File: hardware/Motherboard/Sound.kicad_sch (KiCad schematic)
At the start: 2 parts, among them U29 74LS02, U65 AY-3-8910A

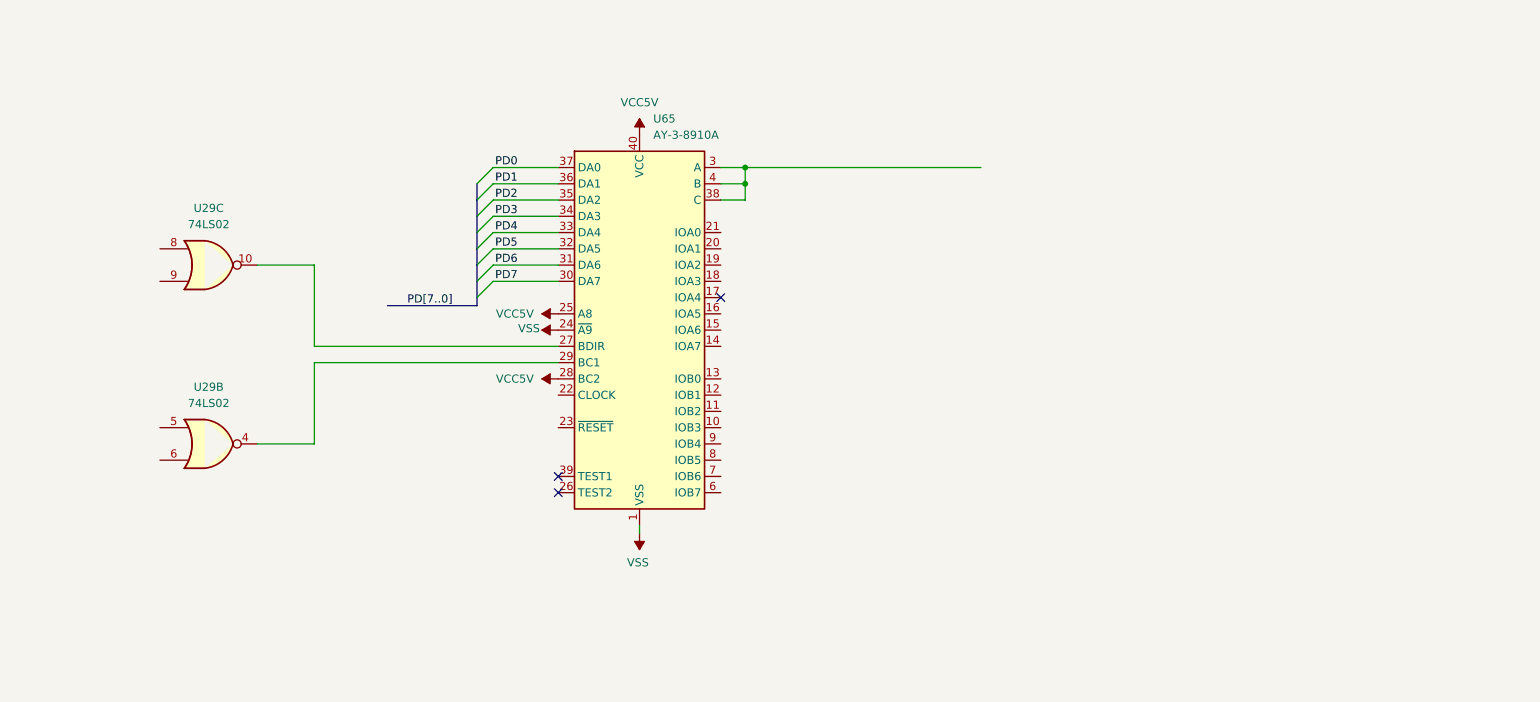
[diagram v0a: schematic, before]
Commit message: WIP
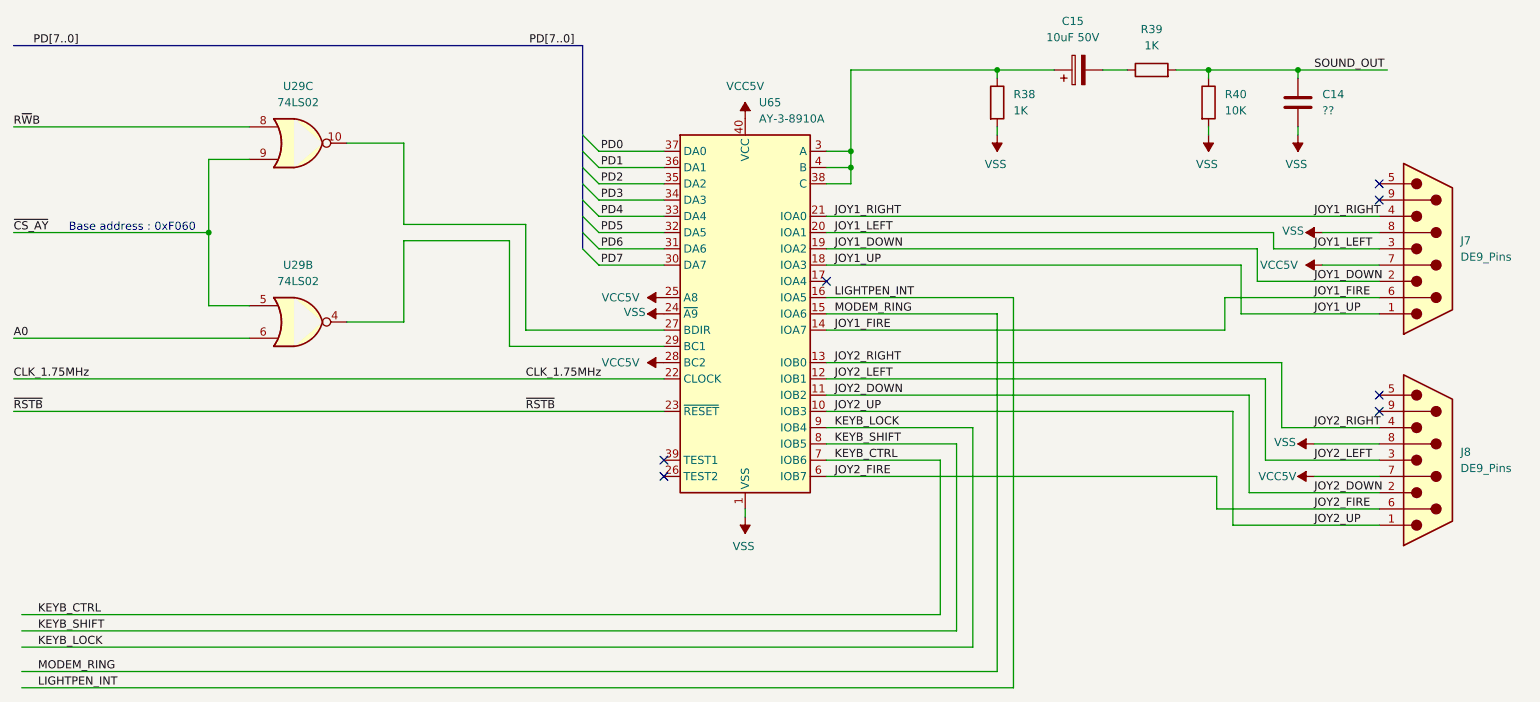
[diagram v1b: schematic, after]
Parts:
- added C14: ??, symbol Device:C
- added C15: 10uF 50V, symbol Device:C_Polarized
- added J7, J8: DE9_Pins, symbol Connector:DE9_Pins
- added R38, R39: 1K, symbol Device:R
- added R40: 10K, symbol Device:R
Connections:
- net VCC5V: now also J7.7, J8.7
- net VSS: now also C14.2, J7.8, J8.8, R38.2, R40.2
- net JOY2_UP: now reaches U65.10 (IOB3)
- net JOY2_UP: now also J8.1
- net JOY2_DOWN: now reaches U65.11 (IOB2)
- net JOY2_DOWN: now also J8.2
- net JOY2_LEFT: now reaches U65.12 (IOB1)
- net JOY2_LEFT: now also J8.3
- net JOY2_RIGHT: now reaches U65.13 (IOB0)
- net JOY2_RIGHT: now also J8.4
- net JOY1_FIRE: now reaches U65.14 (IOA7)
- net JOY1_FIRE: now also J7.6
- net MODEM_RING: now reaches U65.15 (IOA6)
- net LIGHTPEN_INT: now reaches U65.16 (IOA5)
- net JOY1_UP: now reaches U65.18 (IOA3)
- net JOY1_UP: now also J7.1
- net JOY1_DOWN: now reaches U65.19 (IOA2)
- net JOY1_DOWN: now also J7.2
- net JOY1_LEFT: now reaches U65.20 (IOA1)
- net JOY1_LEFT: now also J7.3
- net JOY1_RIGHT: now reaches U65.21 (IOA0)
- net JOY1_RIGHT: now also J7.4
- net CLK_1.75MHz: now reaches U65.22 (CLOCK)
- net ~{RSTB}: now reaches U65.23 (~{RESET})
- net at U65.3 (A), U65.38 (C), U65.4 (B): now also C15.1, R38.1
- net JOY2_FIRE: now reaches U65.6 (IOB7)
- net JOY2_FIRE: now also J8.6
- net KEYB_CTRL: now reaches U65.7 (IOB6)
- net KEYB_SHIFT: now reaches U65.8 (IOB5)
- net KEYB_LOCK: now reaches U65.9 (IOB4)
- net ~{CS_AY}: now reaches U29.5
- net ~{CS_AY}: now also U29.9
- net A0: now reaches U29.6
- net R~{W}B: now reaches U29.8
- new net: C15.2, R39.1
- new net SOUND_OUT: C14.1, R39.2, R40.1
- no-connect marks 3 -> 7
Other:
- note added: "Base address : 0xF060"
- moved on the sheet: U29B, U29C, U65

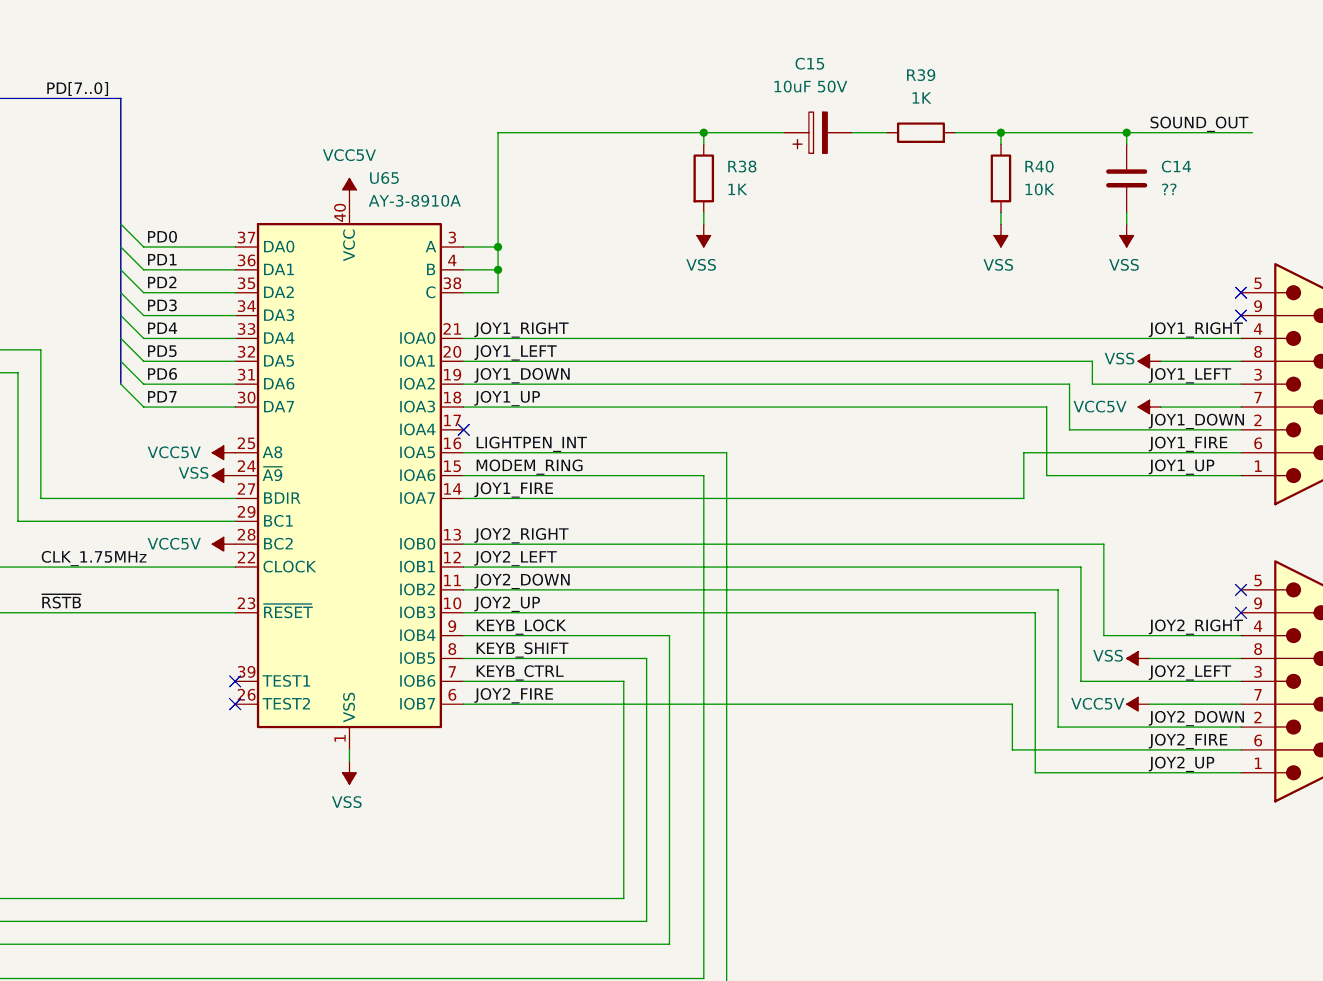
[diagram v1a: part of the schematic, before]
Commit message: WIP
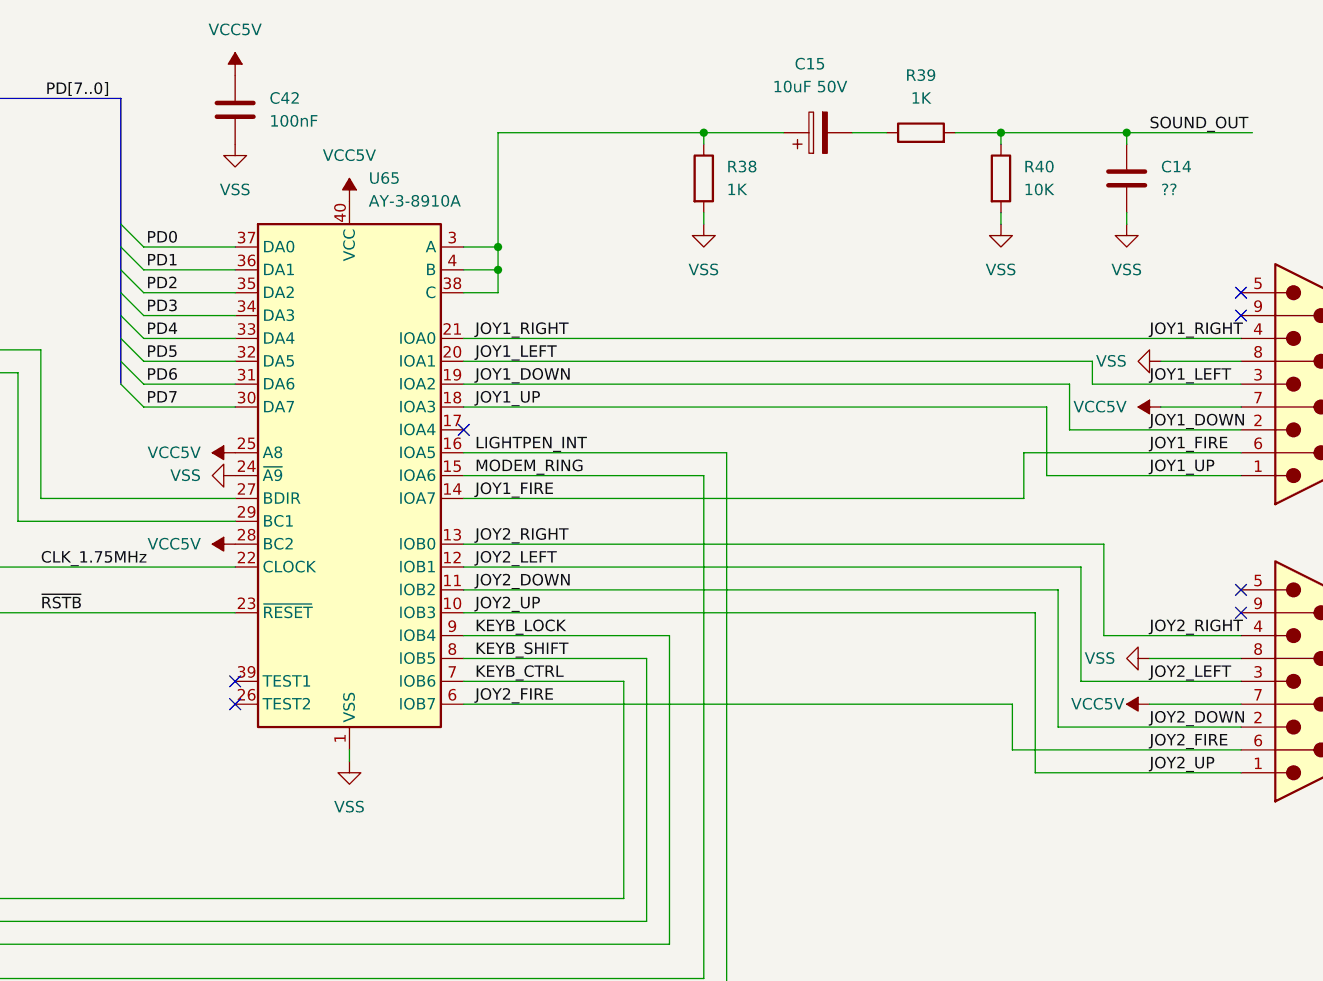
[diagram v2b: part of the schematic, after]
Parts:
- added C42: 100nF, symbol Device:C
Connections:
- net VCC5V: now also C42.1
- net VSS: now also C42.2

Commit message: WIP
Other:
- title: (none) -> Apollo 7 Squale - Sound and joysticks
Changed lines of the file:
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@@
 	(generator_version "9.0")
 	(paper "A4")
+	(title_block
+		(title "Apollo 7 Squale - Sound and joysticks")
+		(rev "0.1")
+		(comment 1 "http://hxc2001.free.fr/Squale/")
+		(comment 2 "CC-BY Licence (Creative Commons Attribution)")
+		(comment 3 "Drawn by Jean-François DEL NERO")
+	)
 	(text "Base address : 0xF060"
 		(exclude_from_sim no)

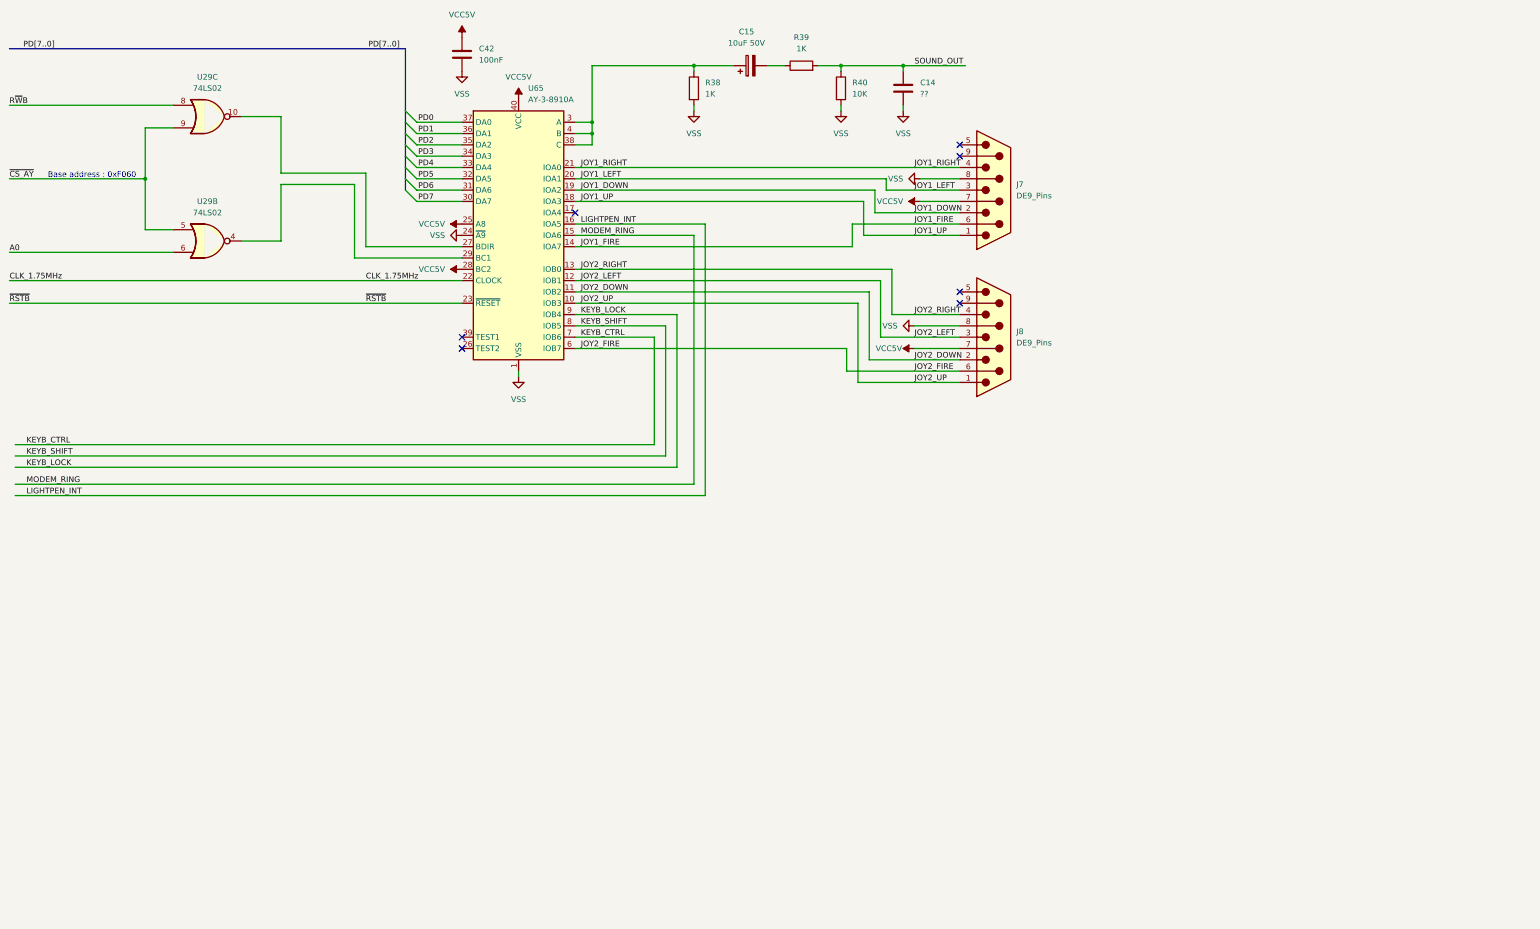
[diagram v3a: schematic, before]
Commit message: WIP.
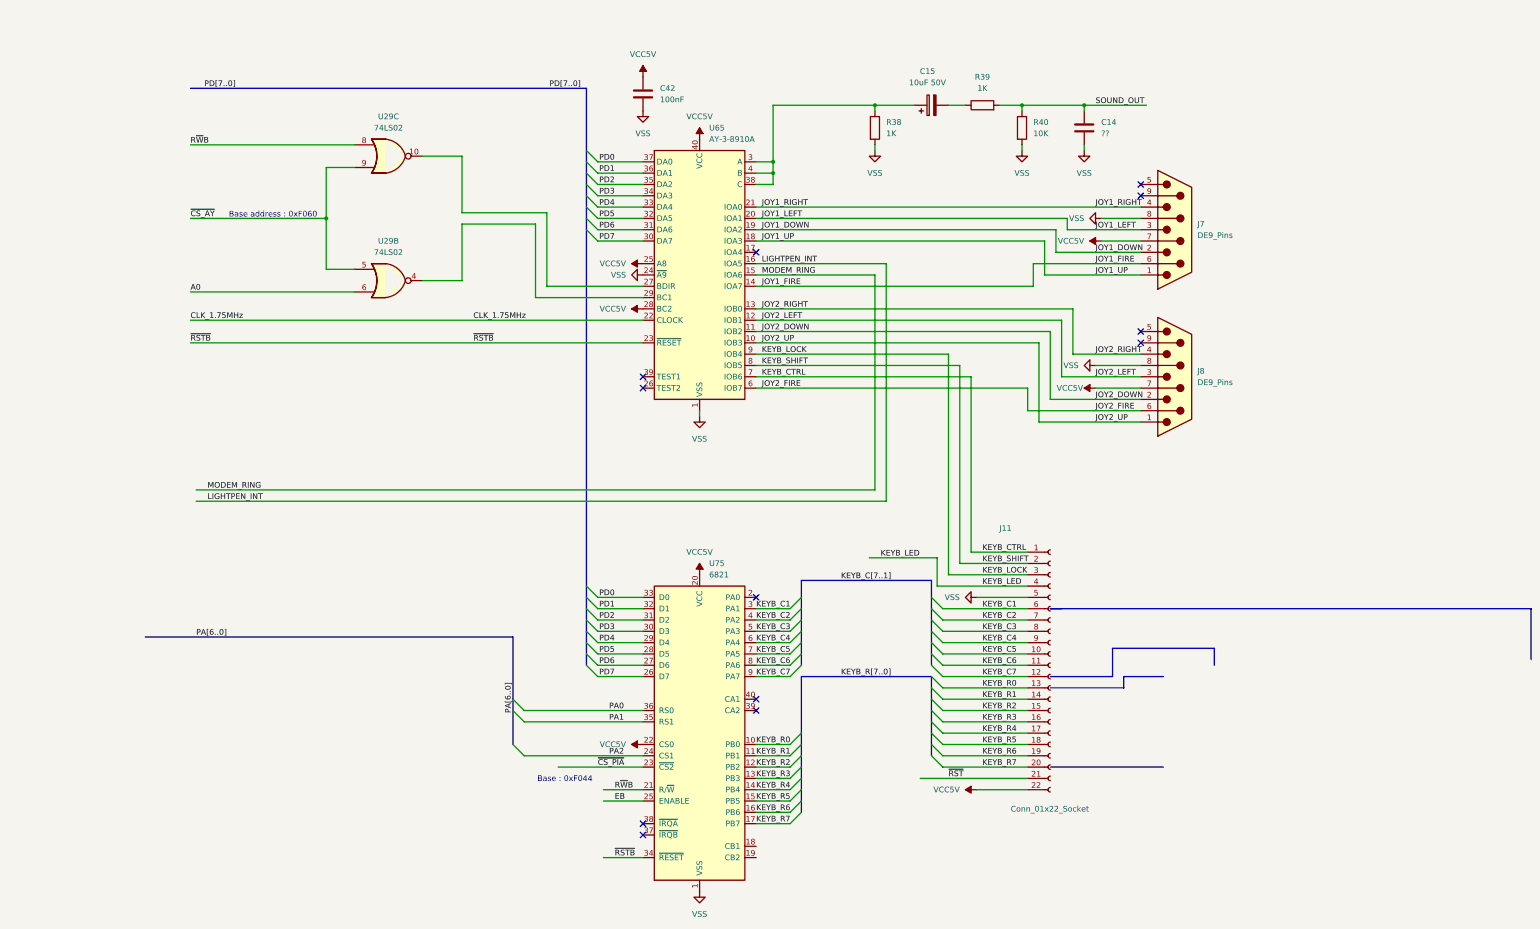
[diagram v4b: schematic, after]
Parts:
- added J11: Conn_01x22_Socket, symbol Connector:Conn_01x22_Socket
- added U75: 6821, Package_DIP:DIP-40_W15.24mm, symbol Interface:6821
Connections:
- net KEYB_CTRL: now also J11.1 (Pin_1)
- net KEYB_LOCK: now also J11.3 (Pin_3)
- net KEYB_SHIFT: now also J11.2 (Pin_2)
- net PD0: now also U75.33 (D0)
- net PD1: now also U75.32 (D1)
- net PD2: now also U75.31 (D2)
- net PD3: now also U75.30 (D3)
- net PD4: now also U75.29 (D4)
- net PD5: now also U75.28 (D5)
- net PD6: now also U75.27 (D6)
- net PD7: now also U75.26 (D7)
- net R~{W}B: now also U75.21 (R/~{W})
- net VCC5V: now also J11.22 (Pin_22), U75.20 (VCC), U75.22 (CS0)
- net VSS: now also J11.5 (Pin_5), U75.1 (VSS)
- net ~{RSTB}: now also U75.34 (~{RESET})
- new net EB: U75.25 (ENABLE)
- new net KEYB_C1: J11.6 (Pin_6), U75.3 (PA1)
- new net KEYB_C2: J11.7 (Pin_7), U75.4 (PA2)
- new net KEYB_C3: J11.8 (Pin_8), U75.5 (PA3)
- new net KEYB_C4: J11.9 (Pin_9), U75.6 (PA4)
- new net KEYB_C5: J11.10 (Pin_10), U75.7 (PA5)
- new net KEYB_C6: J11.11 (Pin_11), U75.8 (PA6)
- new net KEYB_C7: J11.12 (Pin_12), U75.9 (PA7)
- new net KEYB_LED: J11.4 (Pin_4)
- new net KEYB_R0: J11.13 (Pin_13), U75.10 (PB0)
- new net KEYB_R1: J11.14 (Pin_14), U75.11 (PB1)
- new net KEYB_R2: J11.15 (Pin_15), U75.12 (PB2)
- new net KEYB_R3: J11.16 (Pin_16), U75.13 (PB3)
- new net KEYB_R4: J11.17 (Pin_17), U75.14 (PB4)
- new net KEYB_R5: J11.18 (Pin_18), U75.15 (PB5)
- new net KEYB_R6: J11.19 (Pin_19), U75.16 (PB6)
- new net KEYB_R7: J11.20 (Pin_20), U75.17 (PB7)
- new net PA0: U75.36 (RS0)
- new net PA1: U75.35 (RS1)
- new net PA2: U75.24 (CS1)
- new net ~{CS_PIA}: U75.23 (~{CS2})
- new net ~{RST}: J11.21 (Pin_21)
- no-connect marks 7 -> 12
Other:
- note added: "Base : 0xF044"
- moved on the sheet: C14, C15, C42, J7, J8, R38, R39, R40, U29B, U29C, U65
